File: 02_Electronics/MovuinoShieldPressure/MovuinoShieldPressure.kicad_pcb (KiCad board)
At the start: 2 copper layers, 10.5 x 33 mm, 3 parts, among them J2 Rext, J3 DF12-36NOLEGS-MALE

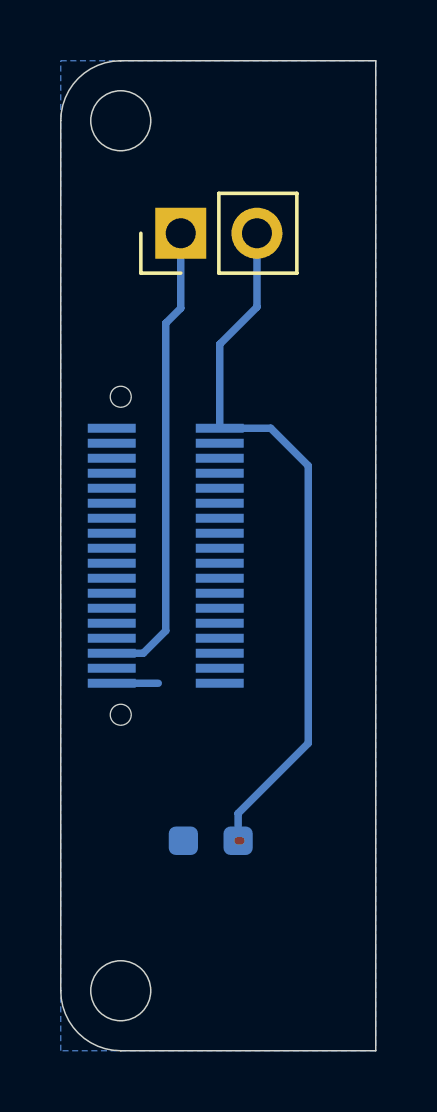
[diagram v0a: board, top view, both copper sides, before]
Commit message: update
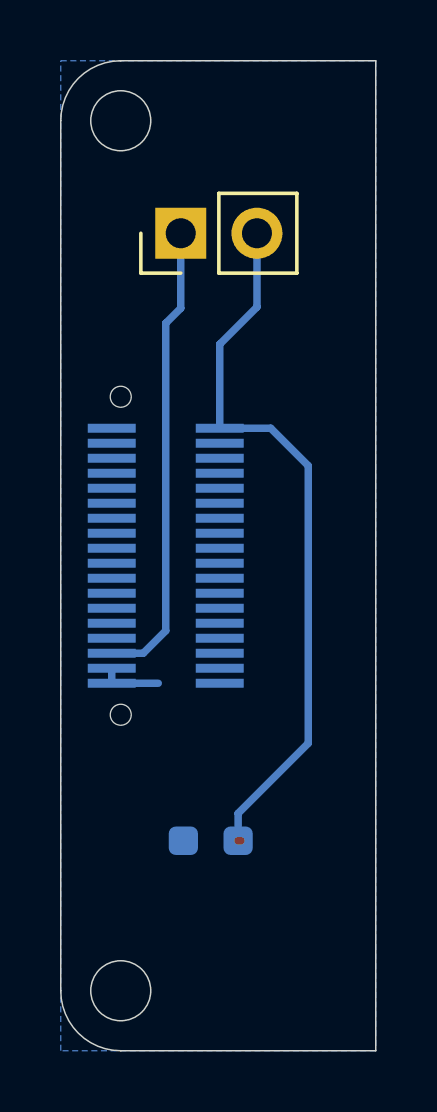
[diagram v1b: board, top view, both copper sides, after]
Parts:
- R1: value Rref -> 330 Ohm
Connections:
- J3 pad 34: Net-(J3-Pad34) -> GND
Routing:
- net GND: track 1.55 -> 2.05 mm
